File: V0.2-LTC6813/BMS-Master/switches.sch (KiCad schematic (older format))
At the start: 15 parts

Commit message: V0.2 LTC6813 block
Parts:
- Q? (x3): symbol Transistor_FET:BSS138 -> BMS-Master-rescue:BSS138-Transistor_FET
- R? (x9): symbol Device:R -> BMS-Master-rescue:R-Device
- U? (x3): symbol Isolator:SFH617A-2X009T -> BMS-Master-rescue:SFH617A-2X009T-Isolator
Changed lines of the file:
@@
 Charge
 $Comp
-L Isolator:SFH617A-2X009T U?
+L BMS-Master-rescue:SFH617A-2X009T-Isolator U?
 U 1 1 5ACC44C1
 P 5150 1950
@@
 $EndComp
 $Comp
-L Isolator:SFH617A-2X009T U?
+L BMS-Master-rescue:SFH617A-2X009T-Isolator U?
 U 1 1 5ACC48D9
 P 5150 4150
@@
 $EndComp
 $Comp
-L Isolator:SFH617A-2X009T U?
+L BMS-Master-rescue:SFH617A-2X009T-Isolator U?
 U 1 1 5ACC490F
 P 5150 5600
@@
 Connection ~ 5850 4050
 $Comp
-L power:+3.3V #PWR?
+L BMS-Master-rescue:+3.3V-power #PWR?
 U 1 1 5ACFE468
 P 4550 1500
@@
 	4550 1850 4850 1850
 $Comp
-L power:+3.3V #PWR?
+L BMS-Master-rescue:+3.3V-power #PWR?
 U 1 1 5ACFE5C5
 P 4600 3850
@@
 	4600 4050 4850 4050
 $Comp
-L power:+3.3V #PWR?
+L BMS-Master-rescue:+3.3V-power #PWR?
 U 1 1 5ACFE760
 P 4550 5250
@@
 	4550 5500 4850 5500
 $Comp
-L Transistor_FET:BSS138 Q?
+L BMS-Master-rescue:BSS138-Transistor_FET Q?
 U 1 1 5AD010B8
 P 3900 2350
@@
 $EndComp
 $Comp
-L Device:R R?
+L BMS-Master-rescue:R-Device R?
 U 1 1 5AD011B7
 P 4350 2050
@@
 $EndComp
 $Comp
-L Device:R R?
+L BMS-Master-rescue:R-Device R?
 U 1 1 5AD01241
 P 2950 2350
@@
 $EndComp
 $Comp
-L Device:R R?
+L BMS-Master-rescue:R-Device R?
 U 1 1 5AD01290
 P 3400 2550
@@
 	2300 2350 2800 2350
 $Comp
-L power:GND #PWR?
+L BMS-Master-rescue:GND-power #PWR?
 U 1 1 5AD03C7A
 P 3750 2900
@@
 	4000 2050 4000 2150
 $Comp
-L Transistor_FET:BSS138 Q?
+L BMS-Master-rescue:BSS138-Transistor_FET Q?
 U 1 1 5AD06F84
 P 3900 4550
@@
 $EndComp
 $Comp
-L Device:R R?
+L BMS-Master-rescue:R-Device R?
 U 1 1 5AD06F8A
 P 4350 4250
@@
 $EndComp
 $Comp
-L Device:R R?
+L BMS-Master-rescue:R-Device R?
 U 1 1 5AD06F90
 P 2950 4550
@@
 $EndComp
 $Comp
-L Device:R R?
+L BMS-Master-rescue:R-Device R?
 U 1 1 5AD06F96
 P 3400 4750
@@
 	2300 4550 2800 4550
 $Comp
-L power:GND #PWR?
+L BMS-Master-rescue:GND-power #PWR?
 U 1 1 5AD06FA2
 P 3750 5100
@@
 	4000 4250 4000 4350
 $Comp
-L Transistor_FET:BSS138 Q?
+L BMS-Master-rescue:BSS138-Transistor_FET Q?
 U 1 1 5AD07A68
 P 4150 6000
@@
 $EndComp
 $Comp
-L Device:R R?
+L BMS-Master-rescue:R-Device R?
 U 1 1 5AD07A6E
 P 4600 5700
@@
 $EndComp
 $Comp
-L Device:R R?
+L BMS-Master-rescue:R-Device R?
 U 1 1 5AD07A74
 P 3200 6000
@@
 $EndComp
 $Comp
-L Device:R R?
+L BMS-Master-rescue:R-Device R?
 U 1 1 5AD07A7A
 P 3650 6200
@@
 	4250 5700 4450 5700
 $Comp
-L power:GND #PWR?
+L BMS-Master-rescue:GND-power #PWR?
 U 1 1 5AD07A86
 P 4000 6550

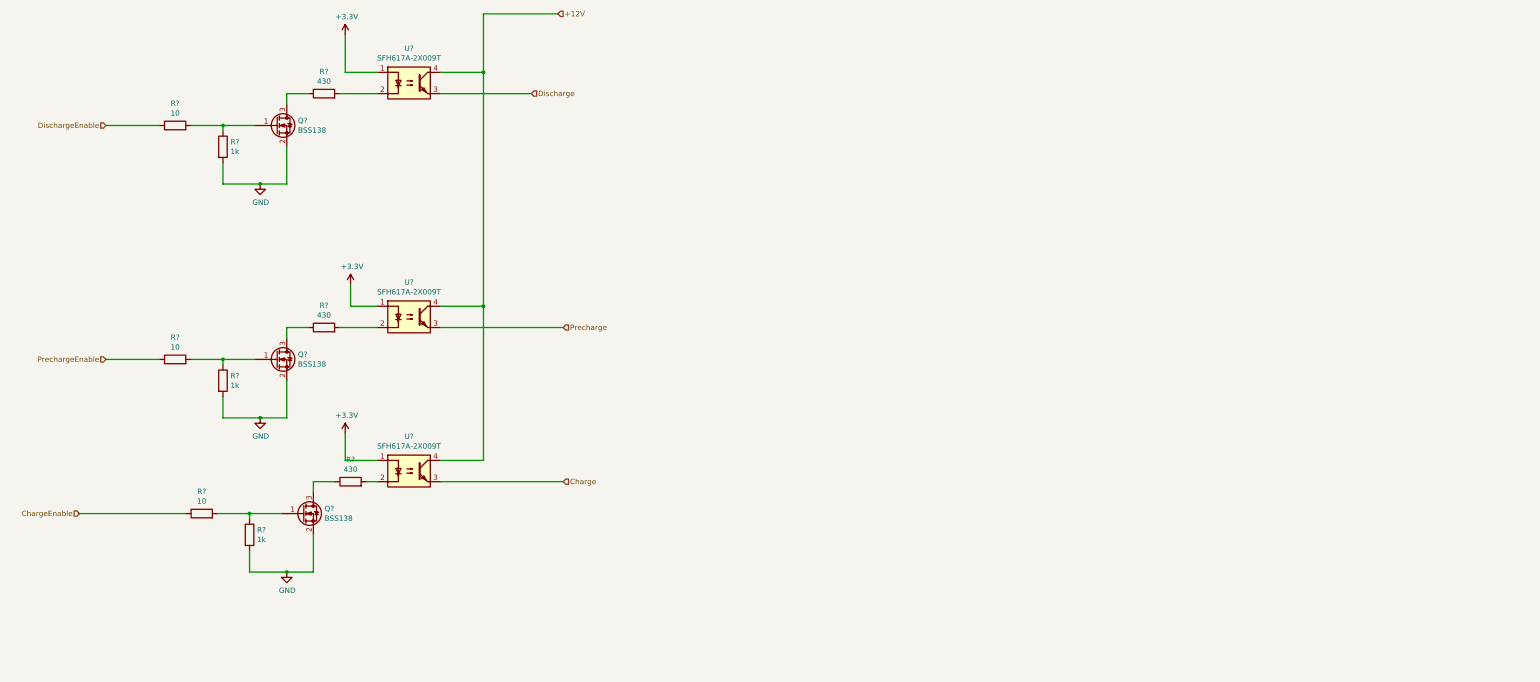
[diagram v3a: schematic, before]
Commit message: Schematics 75% completed
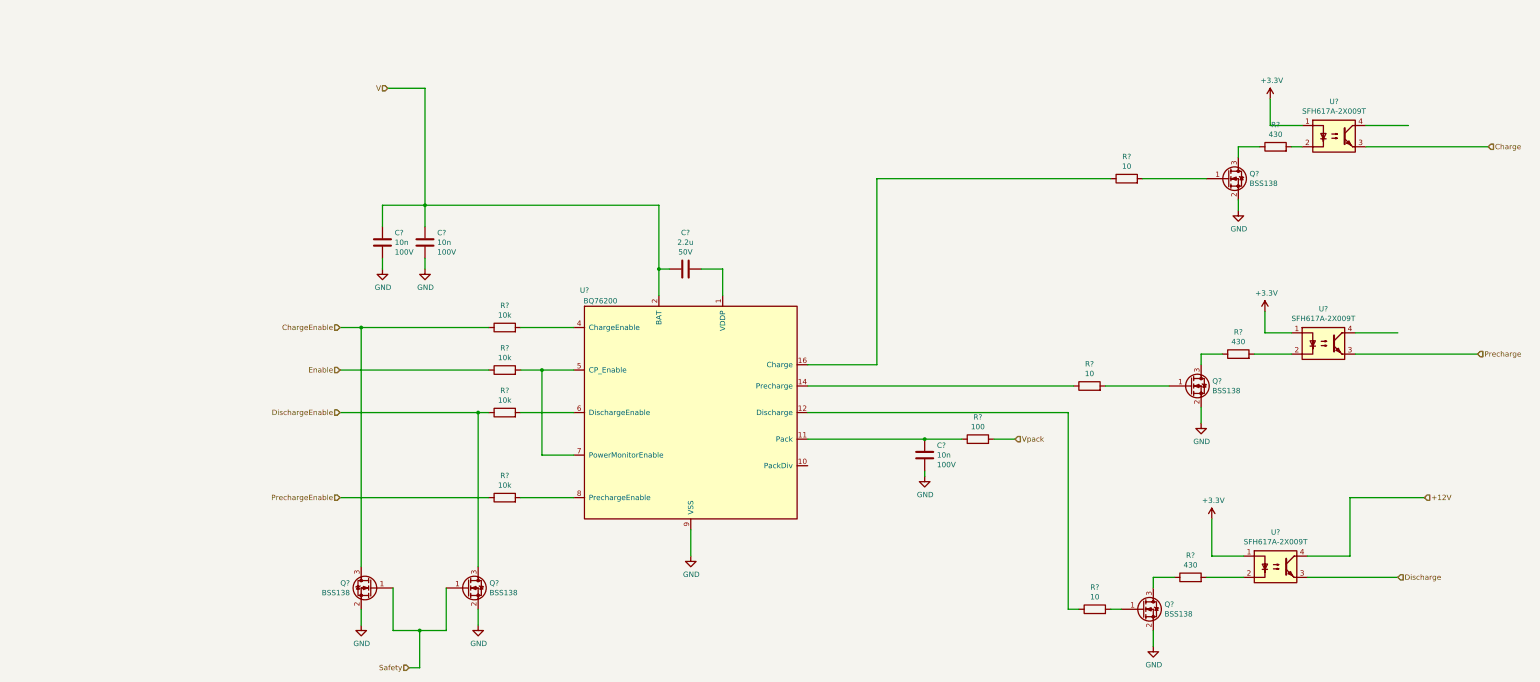
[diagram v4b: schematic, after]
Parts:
- removed R? (x3): 1k, Resistors_SMD:R_0603_HandSoldering, symbol BMS-Master-rescue:R-Device
- added C? (x3): 10n, symbol Device:C
- added C?: 2.2u, symbol Device:C
- added Q? (x2): BSS138, Package_TO_SOT_SMD:SOT-23, symbol Transistor_FET:BSS138
- added R?: 100, Resistors_SMD:R_0603_HandSoldering, symbol BMS-Master-rescue:R-Device
- added R? (x4): 10k, Resistors_SMD:R_0603_HandSoldering, symbol BMS-Master-rescue:R-Device
- added U?: BQ76200, symbol ENNOID:BQ76200
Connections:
- net +12V: no longer U?.4, U?.4
- net ChargeEnable: now also Q?.3 (D), R?.1; no longer R?.1
- net DischargeEnable: now also Q?.3 (D), R?.1; no longer R?.1
- net GND: now also C?.1, C?.1, C?.1, Q?.2 (S), Q?.2 (S), U?.9 (VSS)
- net PrechargeEnable: now also R?.1; no longer R?.1
- new net: R?.1, U?.12 (Discharge)
- new net: R?.1, U?.14 (Precharge)
- new net: R?.1, U?.16 (Charge)
- new net: C?.2, R?.1, U?.11 (Pack)
- new net: C?.1, U?.1 (VDDP)
- new net: R?.2, U?.4 (ChargeEnable)
- new net: R?.2, U?.5 (CP_Enable), U?.7 (PowerMonitorEnable)
- new net: R?.2, U?.6 (DischargeEnable)
- new net: R?.2, U?.8 (PrechargeEnable)
- new net Enable: R?.1
- new net Safety: Q?.1 (G), Q?.1 (G)
- new net V: C?.2, C?.2, C?.2, U?.2 (BAT)
- new net Vpack: R?.2
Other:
- moved on the sheet: Q?, R?, U?
